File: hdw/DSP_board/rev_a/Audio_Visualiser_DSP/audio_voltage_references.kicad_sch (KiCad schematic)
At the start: 10 parts

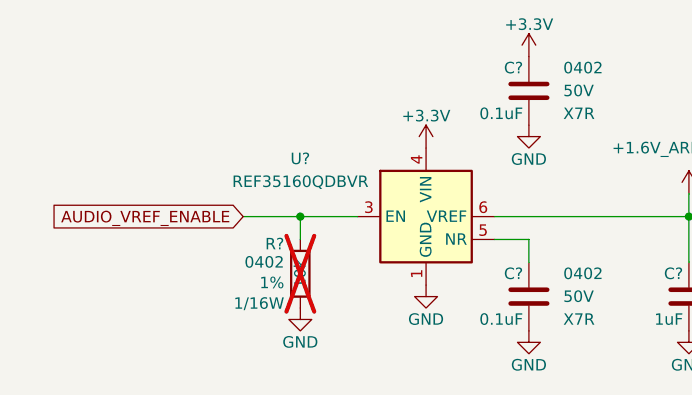
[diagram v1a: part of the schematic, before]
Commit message: more schematic progress
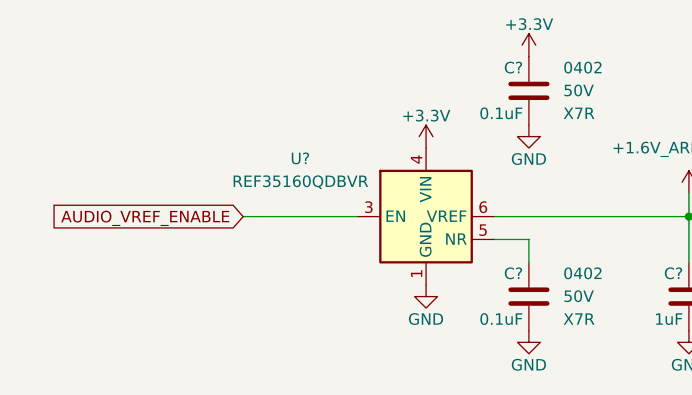
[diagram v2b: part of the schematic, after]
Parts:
- removed R?: 10k, Resistors_SMD:R_0402, symbol Custom_Library:R_Custom
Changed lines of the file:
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@@
-	)
-	(junction
-		(at 119.38 127)
-		(diameter 0)
-		(color 0 0 0 0)
 	)
 	(junction
@@
 	(wire
 		(pts
-			(xy 119.38 127) (xy 125.73 127)
+			(xy 113.03 127) (xy 125.73 127)
 		)
 		(stroke
@@
 	(wire
 		(pts
-			(xy 113.03 127) (xy 119.38 127)
+			(xy 144.78 66.04) (xy 140.97 66.04)
 		)
 		(stroke
@@
 	(wire
 		(pts
-			(xy 144.78 66.04) (xy 140.97 66.04)
-		)
-		(stroke
-			(width 0)
-			(type default)
-		)
-	)
-	(wire
-		(pts
 			(xy 119.38 66.04) (xy 119.38 63.5)
-		)
-		(stroke
-			(width 0)
-			(type default)
-		)
-	)
-	(wire
-		(pts
-			(xy 119.38 129.54) (xy 119.38 127)
 		)
 		(stroke
@@
 	)
 	(symbol
-		(lib_id "power:GND")
-		(at 119.38 137.16 0)
-		(unit 1)
-		(body_style 1)
-		(exclude_from_sim no)
-		(in_bom yes)
-		(on_board yes)
-		(in_pos_files yes)
-		(dnp no)
-		(property "Reference" "#PWR?"
-			(at 119.38 143.51 0)
-			(hide yes)
-			(show_name no)
-			(do_not_autoplace no)
-			(effects
-				(font
-					(size 1.27 1.27)
-				)
-			)
-		)
-		(property "Value" "GND"
-			(at 119.38 140.97 0)
-			(show_name no)
-			(do_not_autoplace no)
-			(effects
-				(font
-					(size 1.27 1.27)
-				)
-			)
-		)
-		(property "Footprint" ""
-			(at 119.38 137.16 0)
-			(hide yes)
-			(show_name no)
-			(do_not_autoplace no)
-			(effects
-				(font
-					(size 1.27 1.27)
-				)
-			)
-		)
-		(property "Datasheet" ""
-			(at 119.38 137.16 0)
-			(hide yes)
-			(show_name no)
-			(do_not_autoplace no)
-			(effects
-				(font
-					(size 1.27 1.27)
-				)
-			)
-		)
-		(property "Description" "Power symbol creates a global label with name \"GND\" , ground"
-			(at 119.38 137.16 0)
-			(hide yes)
-			(show_name no)
-			(do_not_autoplace no)
-			(effects
-				(font
-					(size 1.27 1.27)
-				)
-			)
-		)
-		(pin "1"
-		)
-		(instances
-			(project "Audio_Visualiser_DSP"
-				(path "/97a4dfb8-0e16-46f1-9709-8d2007dd0cd3/6411608b-521a-4c33-acf3-00a911578dd5"
-					(reference "#PWR?")
-					(unit 1)
-				)
-			)
-		)
-	)
-	(symbol
 		(lib_id "power:+3.3V")
 		(at 133.35 55.88 0)
@@
 					(unit 1)
 				)
-			)
-		)
-	)
-	(symbol
-		(lib_id "Custom_Library:R_Custom")
-		(at 119.38 133.35 0)
-		(mirror y)
-		(unit 1)
-		(body_style 1)
-		(exclude_from_sim no)
-		(in_bom yes)
-		(on_board yes)
-		(in_pos_files yes)
-		(dnp yes)
-		(property "Reference" "R?"
-			(at 117.602 130.048 0)
-			(show_name no)
-			(do_not_autoplace no)
-			(effects
-				(font
-					(size 1.27 1.27)
-				)
-				(justify left)
-			)
-		)
-		(property "Value" "10k"
-			(at 119.38 133.35 90)
-			(show_name no)
-			(do_not_autoplace no)
-			(effects
-				(font
-					(size 1.27 1.27)
-				)
-			)
-		)
-		(property "Footprint" "Resistors_SMD:R_0402"
-			(at 119.38 133.35 0)
-			(hide yes)
-			(show_name no)
-			(do_not_autoplace no)
-			(effects
-				(font
-					(size 1.27 1.27)
-				)
-			)
-		)
-		(property "Datasheet" ""
-			(at 119.38 133.35 0)
-			(hide yes)
-			(show_name no)
-			(do_not_autoplace no)
-			(effects
-				(font
-					(size 1.27 1.27)
-				)
-			)
-		)
-		(property "Description" ""
-			(at 119.38 133.35 0)
-			(show_name no)
-			(do_not_autoplace no)
-			(effects
-				(font
-					(size 1.27 1.27)
-				)
-			)
-		)
-		(property "display_footprint" "0402"
-			(at 117.602 132.08 0)
-			(show_name no)
-			(do_not_autoplace no)
-			(effects
-				(font
-					(size 1.27 1.27)
-				)
-				(justify left)
-			)
-		)
-		(property "Tolerance" "1%"
-			(at 117.602 134.366 0)
-			(show_name no)
-			(do_not_autoplace no)
-			(effects
-				(font
-					(size 1.27 1.27)
-				)
-				(justify left)
-			)
-		)
-		(property "Wattage" "1/16W"
-			(at 117.602 136.652 0)
-			(show_name no)
-			(do_not_autoplace no)
-			(effects
-				(font
-					(size 1.27 1.27)
-				)
-				(justify left)
-			)
-		)
-		(property "Digi-Key PN" "541-100KHCT-ND"
-			(at 119.38 133.35 0)
-			(hide yes)
-			(show_name no)
-			(do_not_autoplace no)
-			(effects
-				(font
-					(size 1.27 1.27)
-				)
-			)
-		)
-		(pin "1"
-		)
-		(pin "2"
-		)
-		(instances
-			(project "Audio_Visualiser_DSP"
-				(path "/97a4dfb8-0e16-46f1-9709-8d2007dd0cd3/6411608b-521a-4c33-acf3-00a911578dd5"
-					(reference "R?")
-					(unit 1)
-				)
